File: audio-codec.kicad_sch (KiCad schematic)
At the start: 21 parts, among them J1 AudioJack2_Ground, J2 AudioJack2_Ground, U4 XTAC5112IRGER

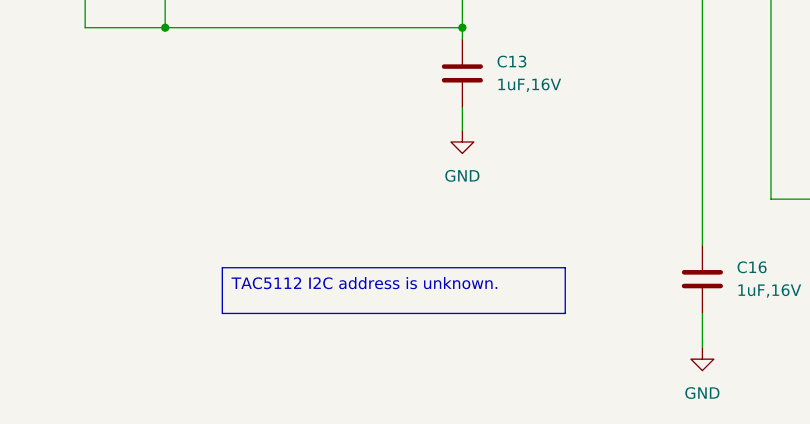
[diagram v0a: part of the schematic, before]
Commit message: remove TS
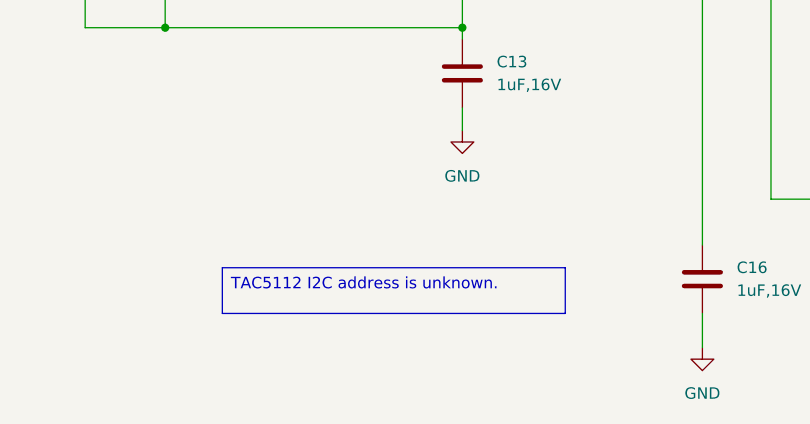
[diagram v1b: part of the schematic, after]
